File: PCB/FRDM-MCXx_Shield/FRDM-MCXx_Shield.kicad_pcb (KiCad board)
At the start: 4 copper layers, 91.4 x 54.6 mm, 56 parts, among them J2 Barrel_Jack_Switch, J3 Conn_01x04_Socket, J4 Conn_01x05_Socket, J5 Conn_01x06_Socket, M1 Motor_Servo, Q1 IRLML6401, SW1 PEC11L-4120F-N0020, SW2 SW_Push, U1 M95010-RMN6TP, U2 FXLS8974CF, U3 SHT31A-DIS, U5 SN74LV164ADR

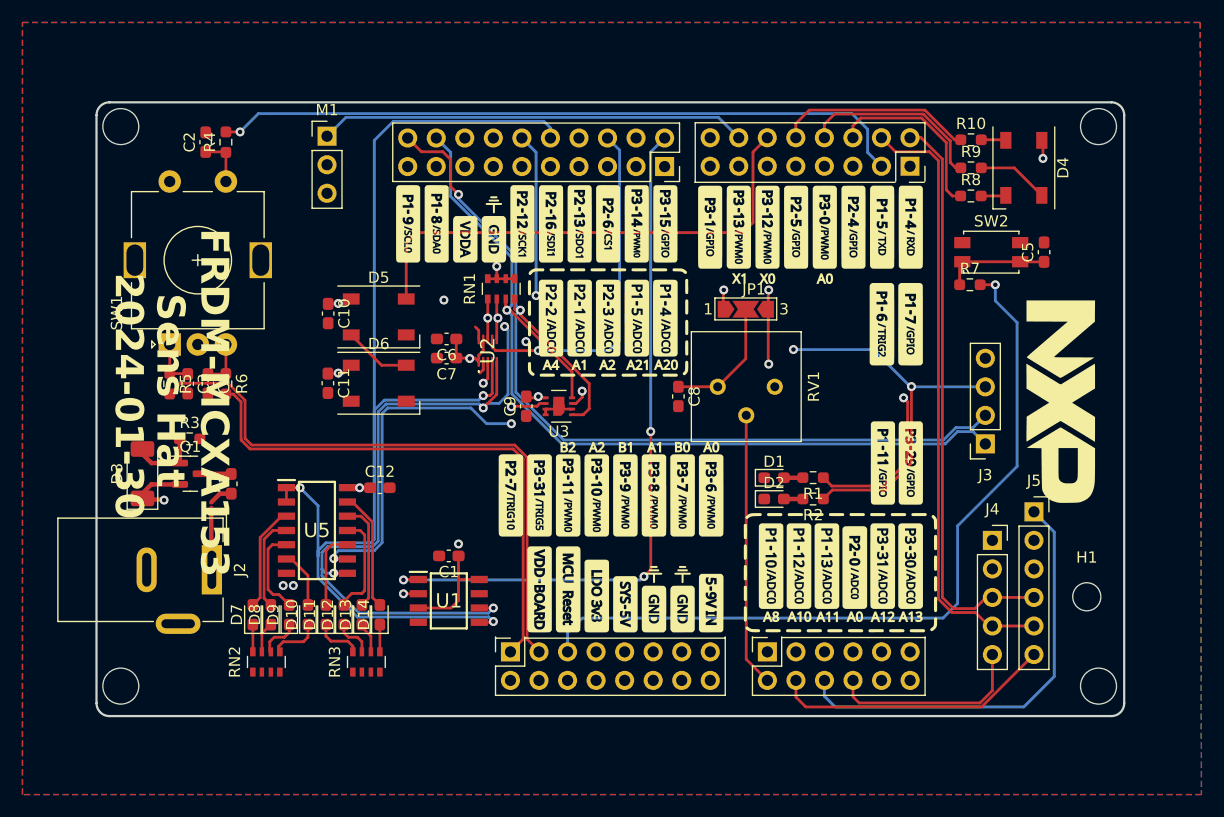
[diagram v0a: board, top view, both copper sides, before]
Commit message: Updated PCB
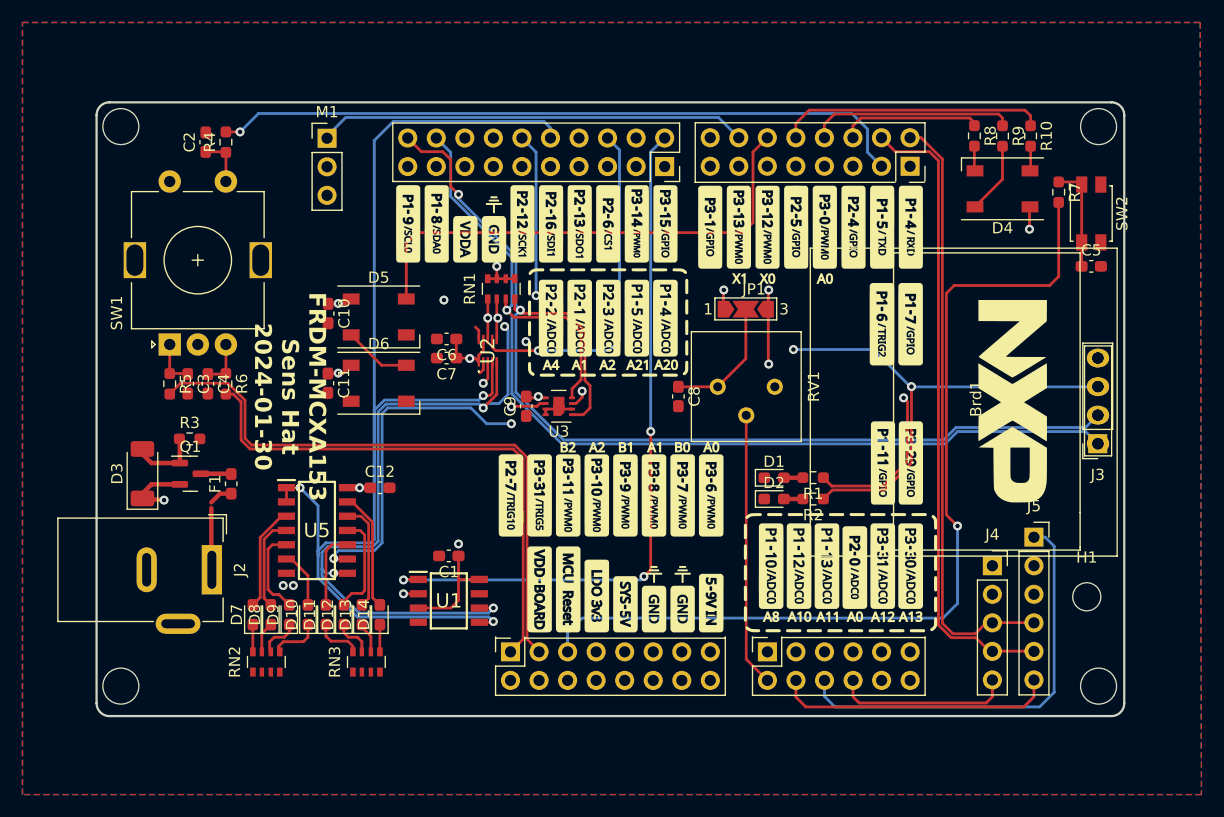
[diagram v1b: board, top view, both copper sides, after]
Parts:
- added ?: , clipboard:5e83e988-b69c-43c0-b382-9b895c3e7185, F.Cu at (187.2, 91.1)
- added Brd1: SSD1306, OLED:128x64OLED, F.Cu at (182.7, 85.5)
- moved R7 11.4 mm to (189.8, 67.1), turned to -90 degrees
- moved J3 10.0 mm to (193.3, 89.5)
- moved SW2 9.54 mm to (192.7, 69.0), turned to -90 degrees
- moved R8 5.36 mm to (182.3, 62.1), turned to -90 degrees
- moved R10 5.31 mm to (187.3, 62.1), turned to -90 degrees
- moved C5 4.39 mm to (192.7, 73.7), turned to 0 degrees
- moved R9 3.99 mm to (184.8, 62.1), turned to -90 degrees
- moved D4 2.66 mm to (184.8, 66.8), turned to 180 degrees
- moved J4 2.26 mm to (183.9, 100.3)
- moved J5 2.26 mm to (187.6, 97.8)
- moved M1 0.18 mm to (124.7, 62.3)
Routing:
- net +5V: track 148.5 -> 169.1 mm
- net /SDA: track 82.4 -> 95.6 mm
- net /SWITCH: track 70.2 -> 82.7 mm
- net /SCL: track 87.0 -> 99.4 mm
- net /LED_B: track 17.5 -> 23.7 mm
- net /LED_R: track 16.3 -> 12.6 mm
- net /TX: track 54.4 -> 56.7 mm
- net /RX: track 51.7 -> 53.9 mm
- net /GPS_PPS: track 17.8 -> 15.8 mm
- net /LED_G: track 16.8 -> 18.3 mm
- net +3.3V: track 316.2 -> 317.1 mm
- net /BT_EN: track 38.8 -> 37.9 mm
- added copper zone on In1.Cu, net GND
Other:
- board text added: "FRDM-MCXA153 Sens Hat 2024-01-30"
